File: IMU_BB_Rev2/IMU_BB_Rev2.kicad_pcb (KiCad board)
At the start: 4 copper layers, 13 x 8 mm, 6 parts, among them J1 Conn_01x04, U1 BMI270

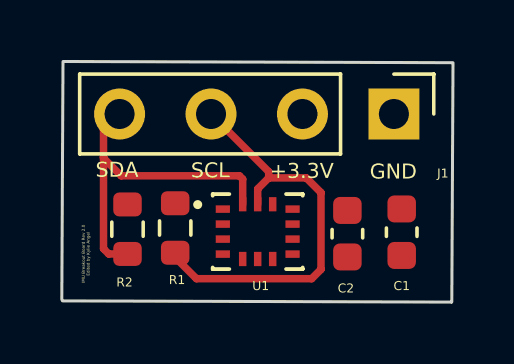
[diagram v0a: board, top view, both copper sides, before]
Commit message: 3/19
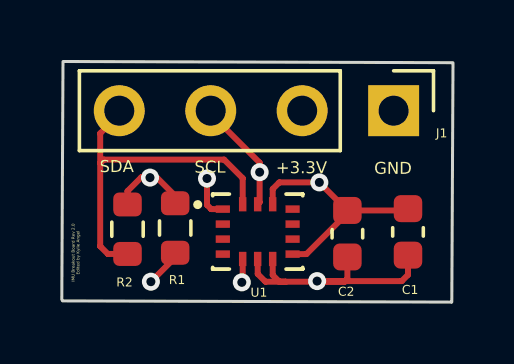
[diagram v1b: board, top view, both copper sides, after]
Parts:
- moved C1 0.21 mm to (79.5, 61.6)
- moved J1 0.11 mm to (79.0, 57.6)
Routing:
- net GND: track 0.00 -> 11.8 mm, vias 0 -> 2
- net +3V3: track 0.00 -> 11.3 mm, vias 0 -> 3
- net /IMU_A_SCL: track 14.7 -> 12.1 mm, vias 0 -> 2

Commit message: final commit
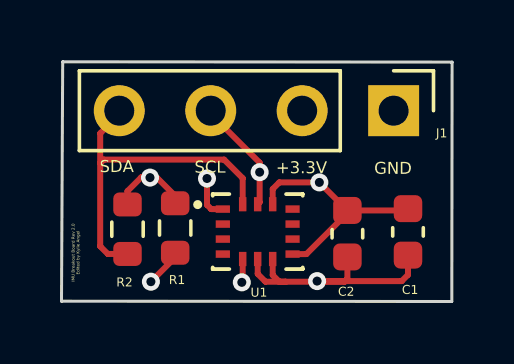
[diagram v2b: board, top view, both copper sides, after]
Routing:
- net /IMU_A_SCL: track 12.1 -> 11.5 mm
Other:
- outline, holes or cut-outs redrawn
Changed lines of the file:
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@@
       (layerselection 0x00010fc_ffffffff)
       (disableapertmacros false)
-      (usegerberextensions false)
+      (usegerberextensions true)
       (usegerberattributes true)
       (usegerberadvancedattributes true)
@@
       (plotinvisibletext false)
       (sketchpadsonfab false)
-      (subtractmaskfromsilk false)
+      (subtractmaskfromsilk true)
       (outputformat 1)
       (mirror false)
-      (drillshape 1)
+      (drillshape 0)
       (scaleselection 1)
-      (outputdirectory "")
+      (outputdirectory "Gerbers_Drill_files/")
     )
   )
@@
       (net 3 "/IMU_A_SDA") (pinfunction "SDX") (pintype "bidirectional"))
   )
-  (gr_line (start 81.03 56.02) (end 80.99 63.96) (layer "Edge.Cuts") (width 0.1))
-  (gr_line (start 68.03 55.94) (end 67.99 63.88) (layer "Edge.Cuts") (width 0.1))
-  (gr_line (start 68.011 63.92) (end 80.969 63.96) (layer "Edge.Cuts") (width 0.1))
-  (gr_line (start 68.072 55.94) (end 81.03 55.98) (layer "Edge.Cuts") (width 0.1))
+  (gr_line (start 81 55.96) (end 80.99 63.94) (layer "Edge.Cuts") (width 0.1))
+  (gr_line (start 68.02 55.95) (end 67.98 63.93) (layer "Edge.Cuts") (width 0.1))
+  (gr_line (start 67.98 63.93) (end 80.99 63.94) (layer "Edge.Cuts") (width 0.1))
+  (gr_line (start 68.02 55.95) (end 81 55.96) (layer "Edge.Cuts") (width 0.1))
   (gr_text "IMU Breakout Board Rev 2.0\nEdited by Kylie Angel" (at 68.45 62.31 90) (layer "F.SilkS")
     (effects (font (size 0.1 0.1) (thickness 0.025)))
@@
   (segment (start 74.585106 59.629859) (end 74.585106 59.311106) (width 0.2) (layer "F.Cu") (net 1))
   (segment (start 74.585106 59.629859) (end 74.585106 60.632394) (width 0.2) (layer "F.Cu") (net 1))
-  (segment (start 72.53 58.124) (end 72.964 57.69) (width 0.25) (layer "F.Cu") (net 1))
+  (segment (start 71.77 62.315) (end 71.77 62.47) (width 0.2) (layer "F.Cu") (net 1))
   (segment (start 74.585106 60.632394) (end 74.52 60.6975) (width 0.2) (layer "F.Cu") (net 1))
-  (segment (start 71.77 62.315) (end 71.77 62.47) (width 0.2) (layer "F.Cu") (net 1))
   (segment (start 74.585106 59.311106) (end 72.964 57.69) (width 0.2) (layer "F.Cu") (net 1))
   (segment (start 71.77 62.47) (end 70.96 63.28) (width 0.2) (layer "F.Cu") (net 1))
   (via (at 70.96 63.28) (size 0.6) (drill 0.3) (layers "F.Cu" "B.Cu") (net 1))
   (via (at 74.585106 59.629859) (size 0.6) (drill 0.3) (layers "F.Cu" "B.Cu") (net 1))
-  (segment (start 71.409511 62.830489) (end 73.619511 62.830489) (width 0.2) (layer "In1.Cu") (net 1))
-  (segment (start 73.619511 62.830489) (end 74.585106 61.864894) (width 0.2) (layer "In1.Cu") (net 1))
-  (segment (start 70.96 63.28) (end 71.409511 62.830489) (width 0.2) (layer "In1.Cu") (net 1))
-  (segment (start 74.585106 61.864894) (end 74.585106 59.629859) (width 0.2) (layer "In1.Cu") (net 1))
+  (segment (start 73.264096 63.18) (end 71.06 63.18) (width 0.2) (layer "In1.Cu") (net 1))
+  (segment (start 71.06 63.18) (end 70.96 63.28) (width 0.2) (layer "In1.Cu") (net 1))
+  (segment (start 73.264096 63.18) (end 74.585106 61.85899) (width 0.2) (layer "In1.Cu") (net 1))
+  (segment (start 74.585106 61.85899) (end 74.585106 59.629859) (width 0.2) (layer "In1.Cu") (net 1))
   (segment (start 70.96 63.28) (end 71 63.24) (width 0.2) (layer "B.Cu") (net 1))
   (segment (start 71.77 60.42) (end 71.77 60.665) (width 0.2) (layer "F.Cu") (net 2))
@@
   (segment (start 77.51 62.455) (end 77.51 63.19) (width 0.2) (layer "F.Cu") (net 4))
   (segment (start 75.44952 63.28048) (end 77.41952 63.28048) (width 0.2) (layer "F.Cu") (net 4))
-  (segment (start 72.83 59.84) (end 72.83 59.71) (width 0.2) (layer "F.Cu") (net 4))
   (via (at 72.83 59.84) (size 0.6) (drill 0.3) (layers "F.Cu" "B.Cu") (net 4))
   (via (at 76.5 63.26) (size 0.6) (drill 0.3) (layers "F.Cu" "B.Cu") (net 4))
